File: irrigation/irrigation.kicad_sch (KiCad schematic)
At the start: 46 parts, among them J1 24V Jmp, J10 24V, J11 25%, J12 50%, J13 75%, J14 100%, J15 100%, J16 100%, J17 Pump, J18 Outlet Pump, J19 Empty, J2 Power, J20 25%, J21 25%, J3 Power, J4 Power, J5 Power, J6 Power, J7 Power, J8 0V Jmp, J9 Empty, K1 PLC-RPT-24DC/21, K2 PLC-RPT-24DC/21, K3 PLC-RPT-24DC/21, K4 PLC-RPT-24DC/21, M1 Well Pump, M2 Outlet Pump, SW1 Well Empty, SW2 100% Full, SW3 25% Full, SW4 50% Full, SW5 75% Full, SW6 Drain Switch, SW7 Fill Switch, U1 MPPT-Charger

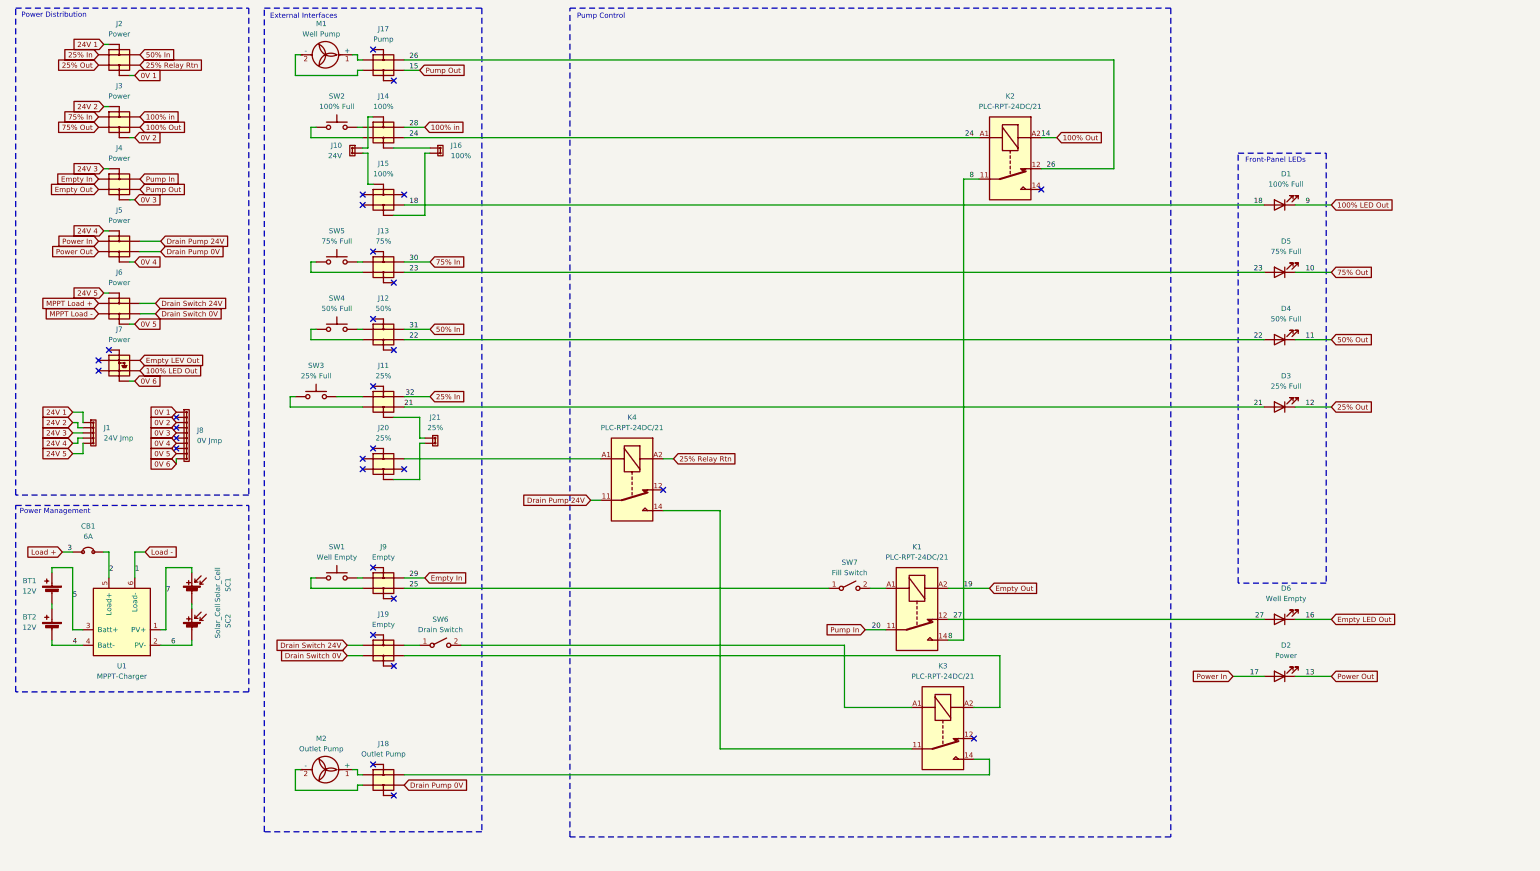
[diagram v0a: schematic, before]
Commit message: Layout
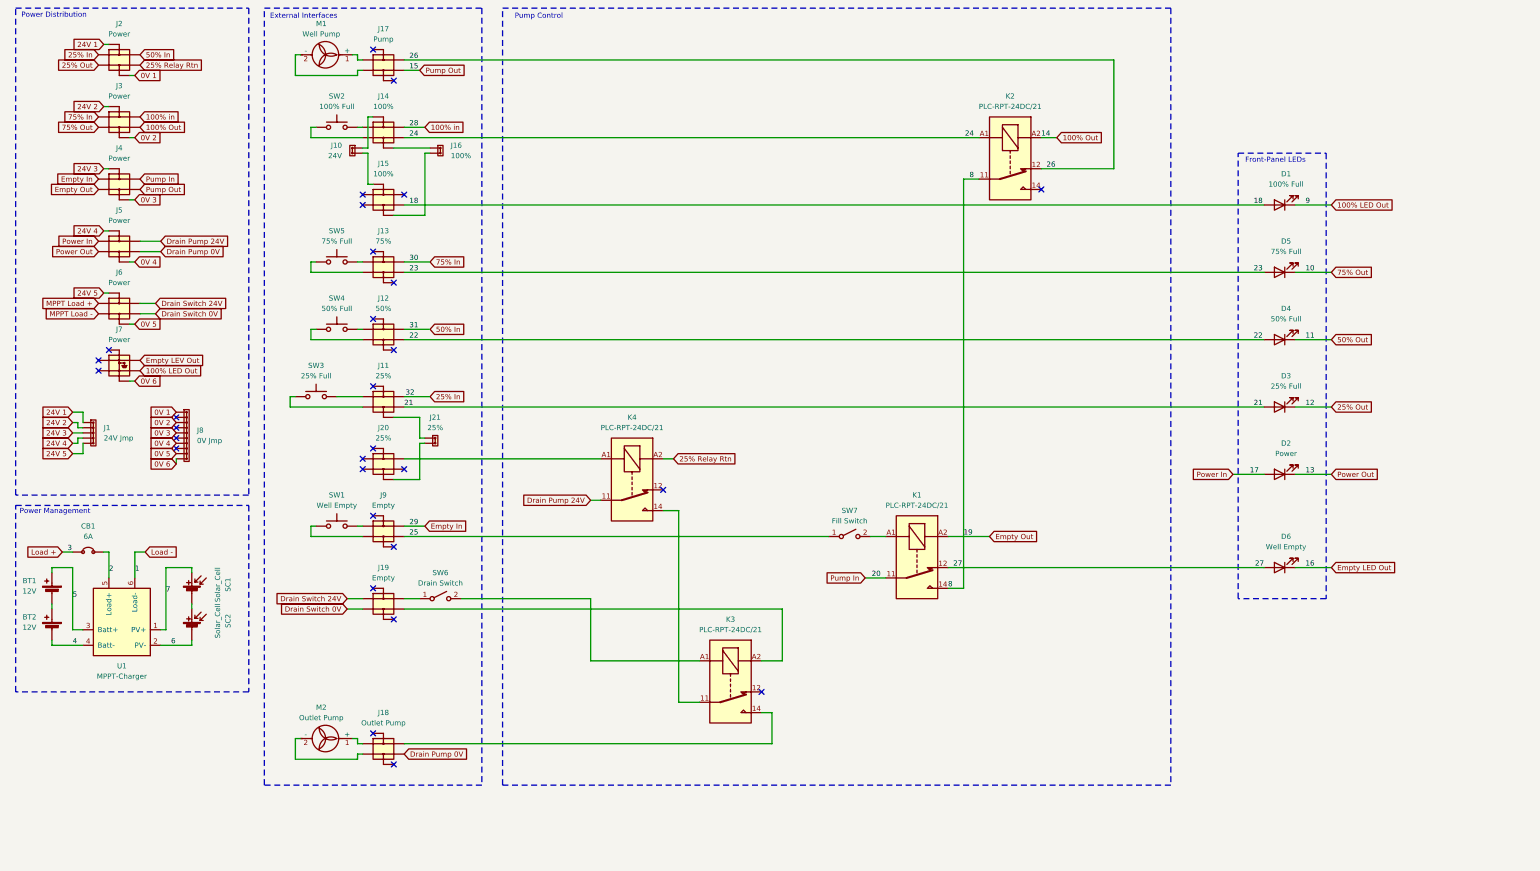
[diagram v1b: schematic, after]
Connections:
- net at J10.: now also J15.; no longer J14.
- net at J16.: now also J15.; no longer J14.
- net at J21.: now also J11.; no longer J20.
- net at J20.: now also K4.A1
- new net: J10., J14.
- new net: J14., J16.
- new net: J20., J21.
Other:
- moved on the sheet: D2, D6, J18, J19, J9, K1, K3, M2, SW1, SW6, SW7

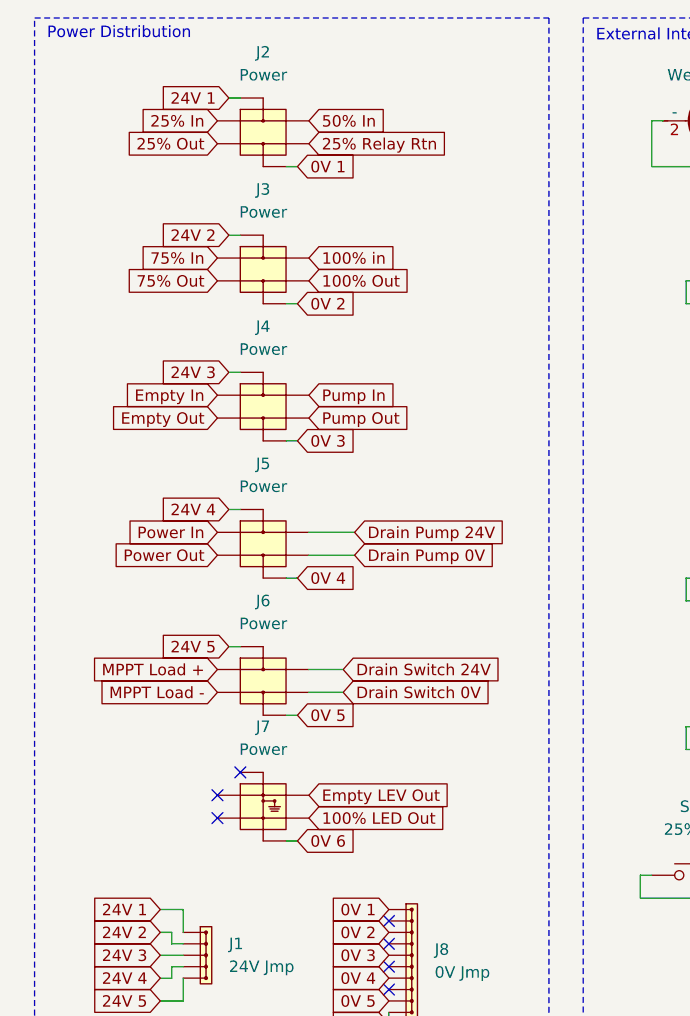
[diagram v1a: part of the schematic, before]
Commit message: More numbers
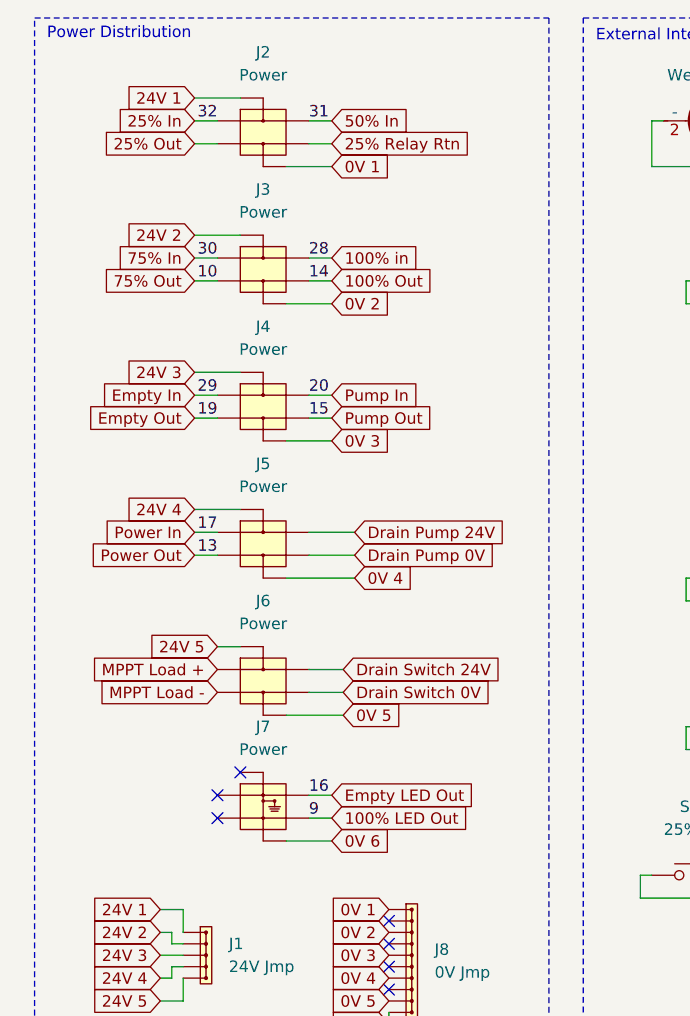
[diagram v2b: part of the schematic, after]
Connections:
- net Empty LEV Out is gone; now on net Empty LED Out: J7.
- net at J10.: now also J15.; no longer J14.
- net at J16.: now also J15.; no longer J14.
- net at J21.: now also J11.; no longer J20.
- net at J20.: now also K4.A1
- new net: J10., J14.
- new net: J14., J16.
- new net: J20., J21.

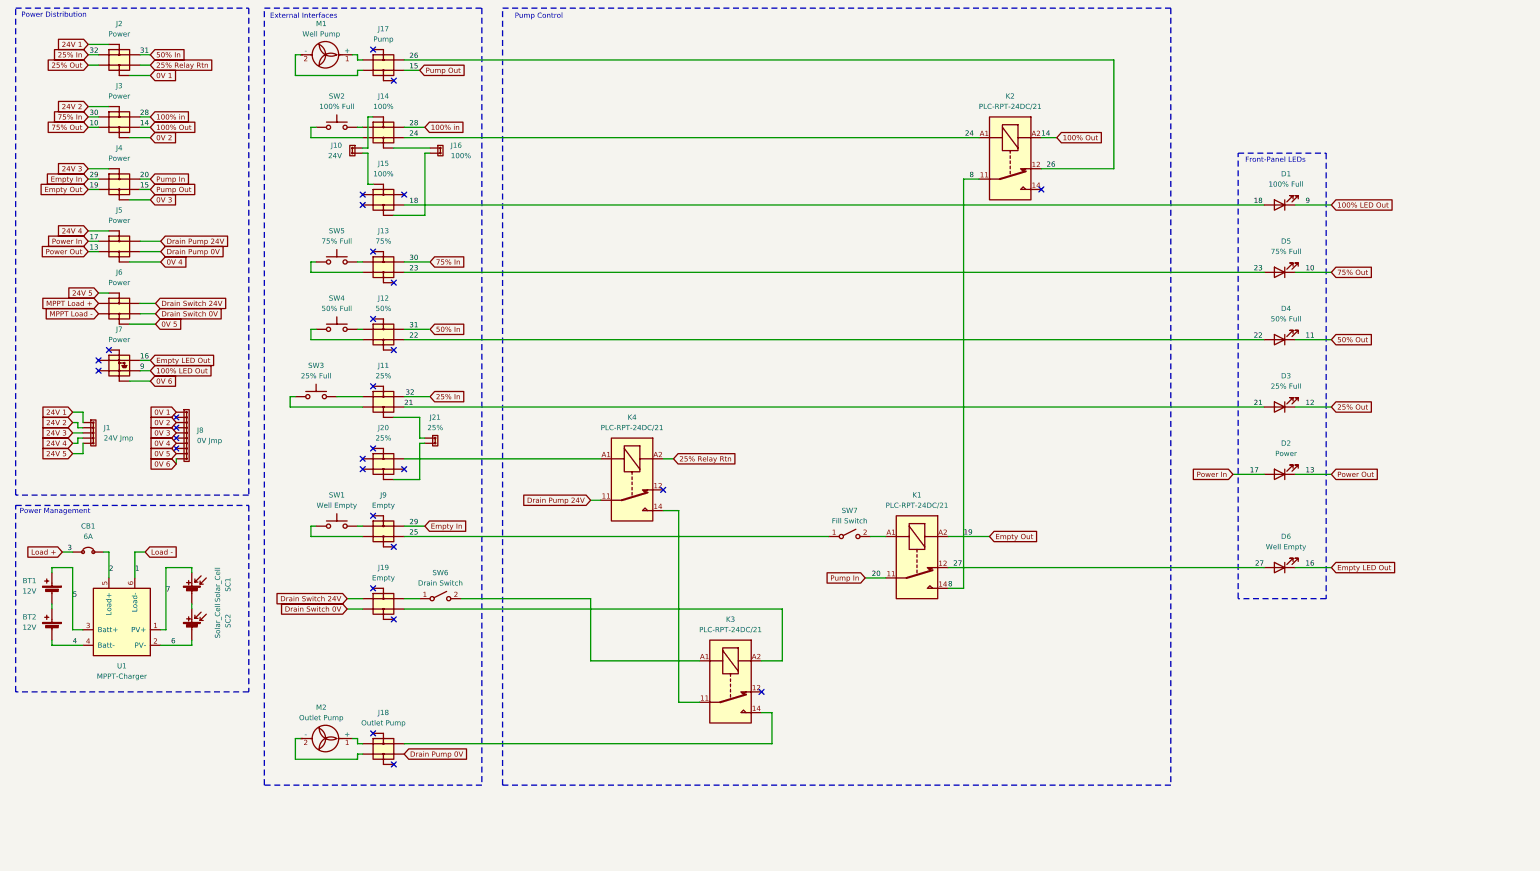
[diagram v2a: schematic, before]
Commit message: Finished updates
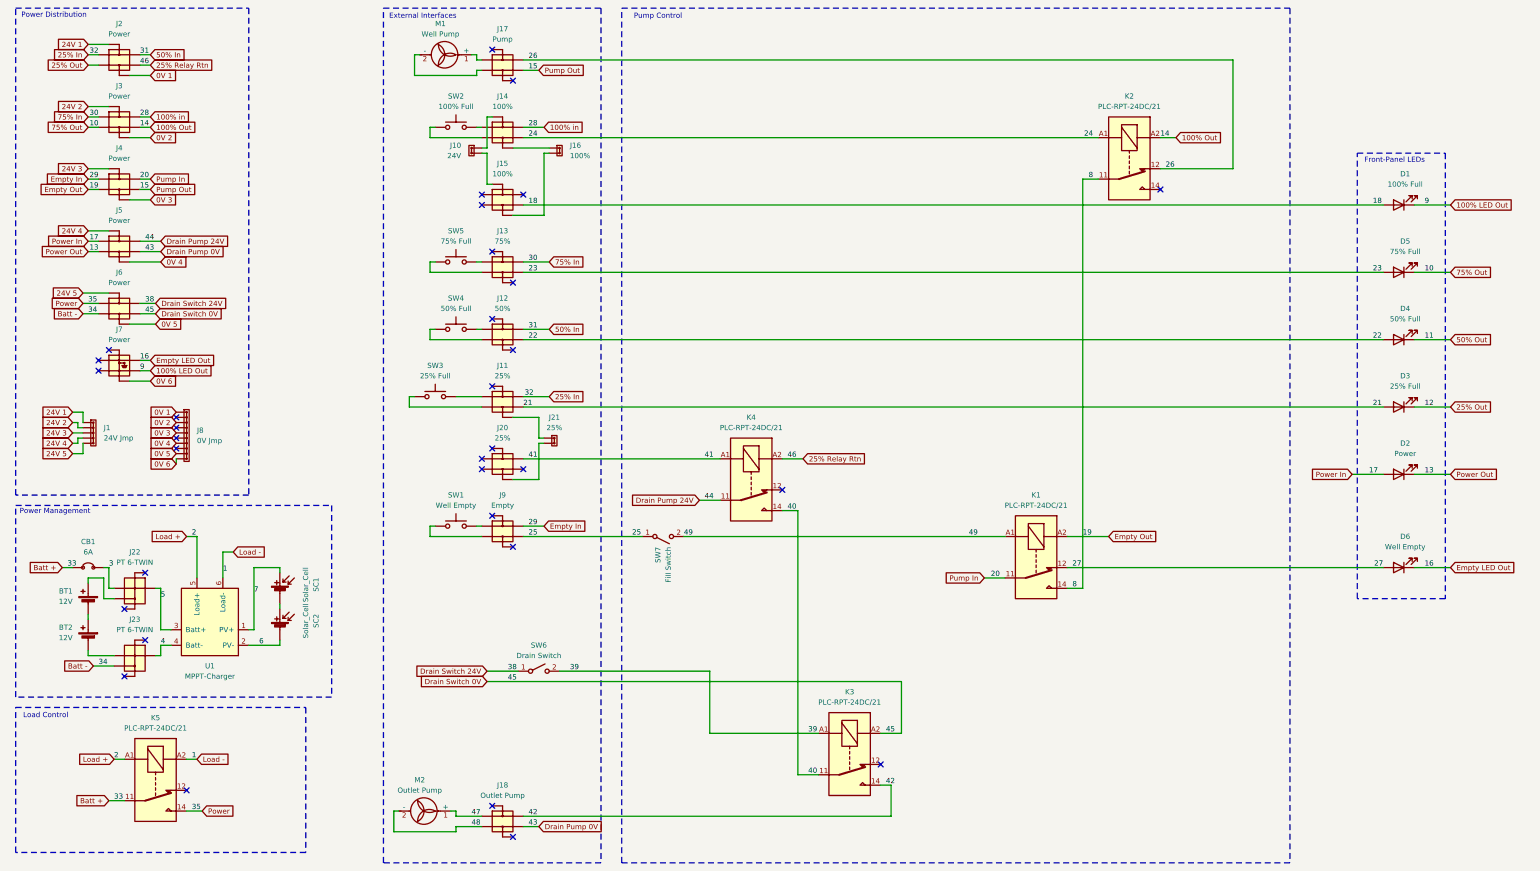
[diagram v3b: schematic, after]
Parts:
- removed J19: Empty, symbol Phoenix Contact:PTTB_2,5-L/N_3210994
- added J22, J23: PT 6-TWIN, symbol Phoenix Contact:PT 6-TWIN
- added K5: PLC-RPT-24DC/21, symbol Phoenix Contact:PLC-RPT-24DC/21
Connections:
- net MPPT Load - is gone; now on net Power: J6.
- net 4: now also J23.; no longer BT2.2 (-)
- net 5: now also J22.; no longer BT1.1 (+)
- net Drain Switch 0V: now also K3.A2
- net Drain Switch 24V: now also SW6.1 (A)
- net Load +: now also U1.5 (Load+), K5.A1; no longer CB1.
- net Load -: now also K5.A2
- net at J10.: now also J15.; no longer J14.
- net at J16.: now also J15.; no longer J14.
- net 40: now reaches K3.11, K4.14
- net 42: now reaches J18., K3.14
- net 39: now reaches K3.A1, SW6.2 (B)
- net 47: now reaches J18., M2.1 (+)
- net 48: now reaches J18., M2.2 (-)
- net at J21.: now also J11.; no longer J20.
- net 49: now reaches K1.A1, SW7.2 (B)
- net 41: now reaches J20.
- net 41: now also K4.A1
- net 2 renamed Batt +
- net Batt +: now also K5.11; no longer U1.5 (Load+)
- net MPPT Load + renamed Power
- net Power: now also K5.14
- new net: J10., J14.
- new net: J14., J16.
- new net: BT2.2 (-), J23.
- new net: BT1.1 (+), J22.
- new net: J20., J21.
- new net 3: CB1., J22.
- new net Batt -: J23., J6.
- no-connect marks 30 -> 33
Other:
- note added: "Load Control"
- moved on the sheet: BT1, BT2, CB1, D1, D2, D3, D4, D5, D6, J10, J11, J12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

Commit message: paper size
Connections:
- net at J10.: now also J15.; no longer J14.
- net at J16.: now also J15.; no longer J14.
- net at J21.: now also J11.; no longer J20.
- new net: J10., J14.
- new net: J14., J16.
- new net: J20., J21.
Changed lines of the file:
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@@
 	(generator "eeschema")
 	(generator_version "9.0")
-	(paper "B")
+	(paper "USLedger")
 	(title_block
 		(title "Irrigation Phase 1")
